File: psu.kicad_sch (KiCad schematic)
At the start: 35 parts, among them J6 Screw_Terminal_01x02, J7 Barrel_Jack_MountingPin, Q1 FDS4435BZ, U1 NCP1117-3.3_SOT223, U6 AP64501SP-13

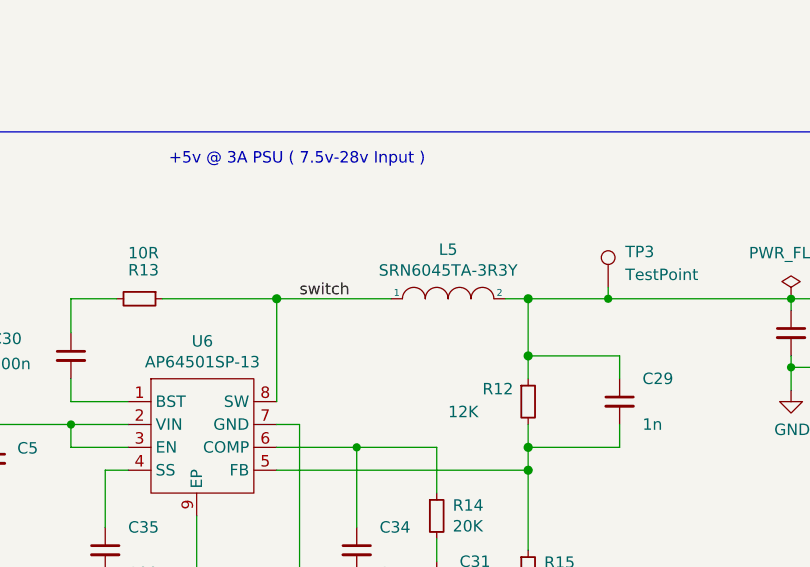
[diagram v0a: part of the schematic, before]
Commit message: Use stadard KiCAD inductor symbol
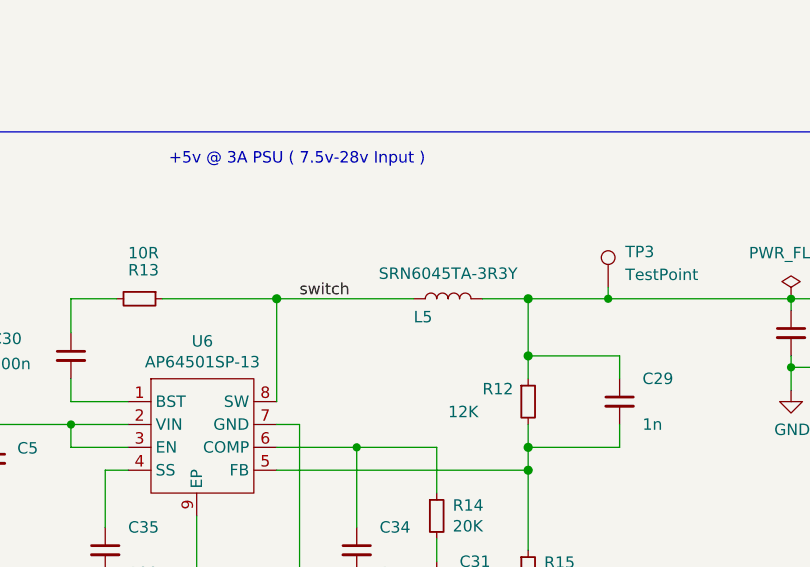
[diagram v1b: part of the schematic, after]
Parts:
- L5: symbol pspice:INDUCTOR -> Device:L
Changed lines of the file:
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@@
-	(wire
-		(pts
-			(xy 170.18 109.22) (xy 172.72 109.22)
-		)
-		(stroke
-			(width 0)
-			(type solid)
-		)
-	)
 	(wire
 		(pts
@@
 		)
 	)
+	(wire
+		(pts
+			(xy 167.64 109.22) (xy 172.72 109.22)
+		)
+		(stroke
+			(width 0)
+			(type default)
+		)
+	)
 	(polyline
 		(pts
@@
 	(wire
 		(pts
-			(xy 144.78 109.22) (xy 157.48 109.22)
+			(xy 144.78 109.22) (xy 160.02 109.22)
 		)
 		(stroke
@@
 	)
 	(symbol
-		(lib_id "pspice:INDUCTOR")
-		(at 163.83 109.22 0)
+		(lib_id "Device:L")
+		(at 163.83 109.22 90)
 		(unit 1)
 		(exclude_from_sim no)
@@
 		(dnp no)
 		(property "Reference" "L5"
-			(at 163.83 103.759 0)
+			(at 161.036 111.252 90)
 			(effects
 				(font
@@
 		)
 		(property "Value" "SRN6045TA-3R3Y"
-			(at 163.83 106.0704 0)
-			(effects
-				(font
+			(at 163.83 106.426 90)
+			(effects
+				(font
